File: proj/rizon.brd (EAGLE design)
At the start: 100 x 80 mm, 41 parts, among them J1 PWRJACK5521, P1 ADDR, P2 DATA, P3 CTL, P4 PWR, P5 10k, U1 Z8400, U10 74273PDIP, U11 74138PDIP, U12 74138PDIP, U13 74138PDIP, U14 74138PDIP, U15 74138PDIP, U16 7432PDIP, U17 74138PDIP, U2 AS6C62256PDIP, U3 AS6C62256PDIP, U4 AT28C64BPLCC, U5 AT28C64BPLCC, U6 7432PDIP, U7 7805TO220, U8 7432PDIP, U9 7400PDIP, X1 OSC412.7

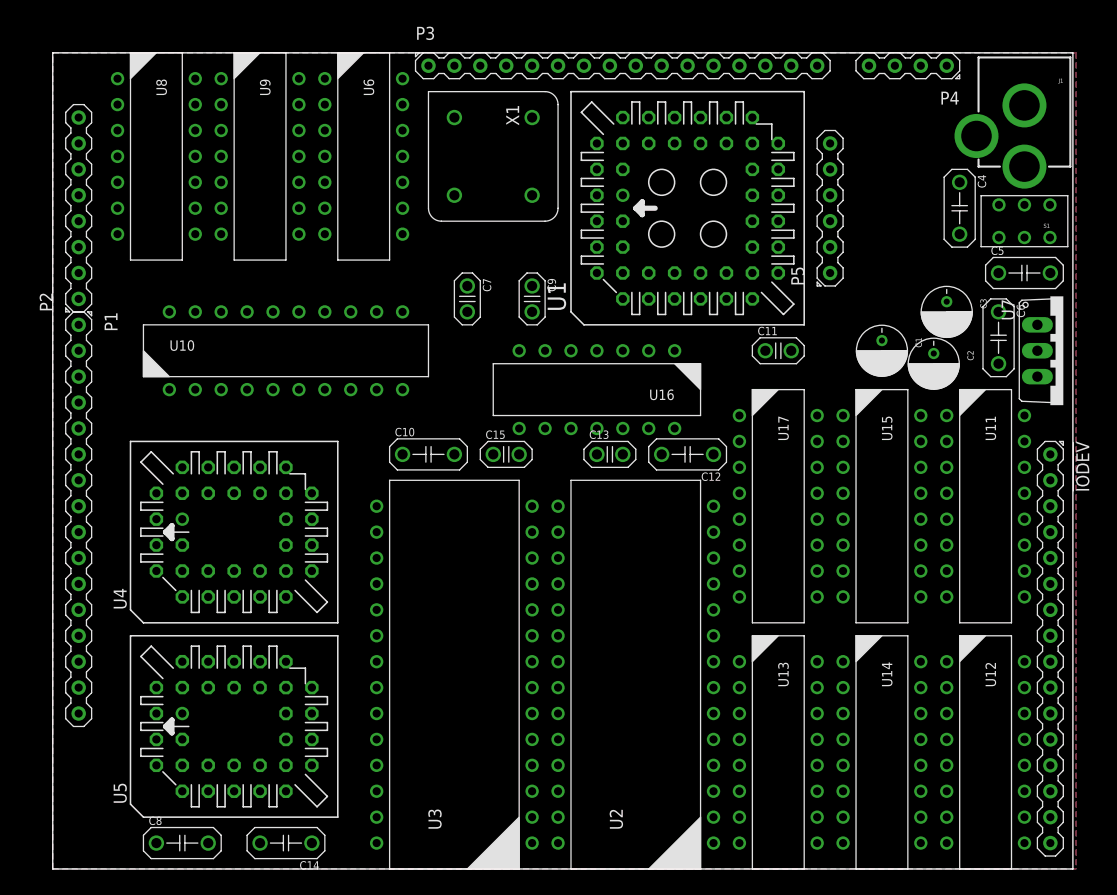
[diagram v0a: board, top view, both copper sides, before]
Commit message: Further designed Rizon board
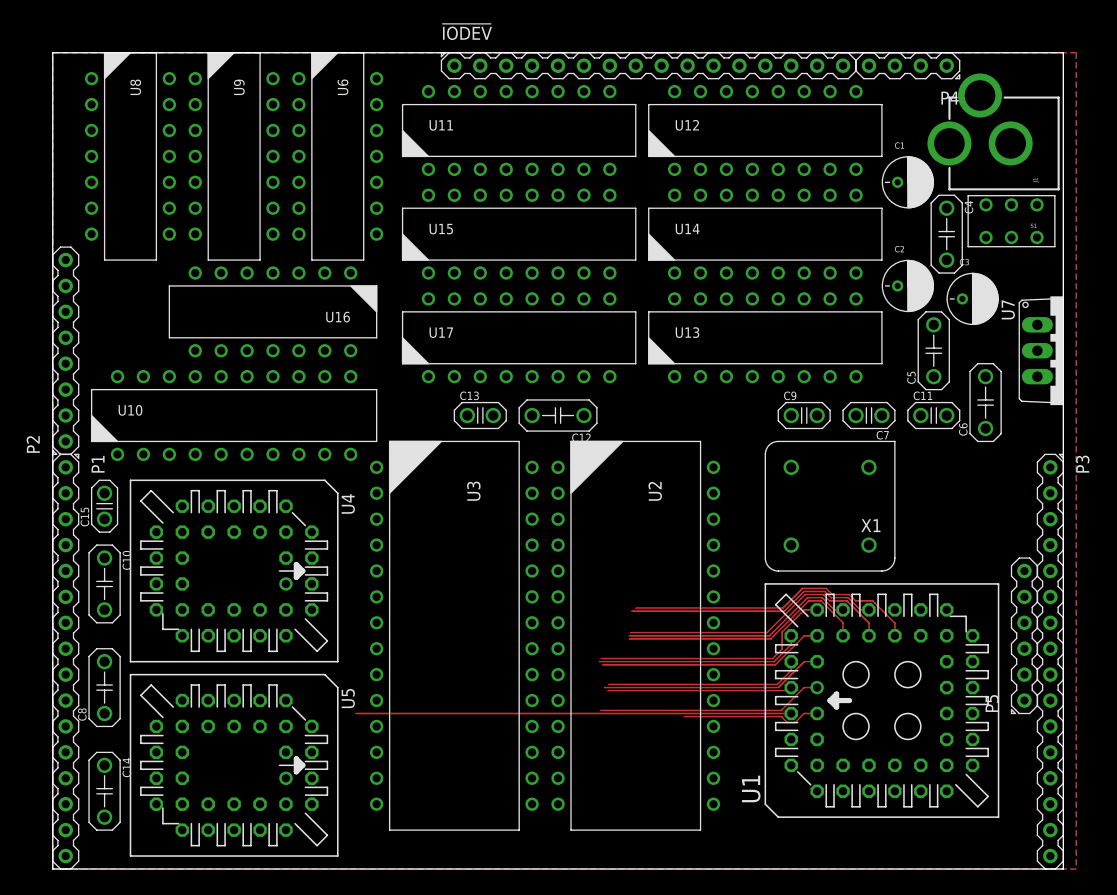
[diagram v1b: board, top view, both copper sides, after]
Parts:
- moved P3 71.9 mm to (97.8, 20.3), turned to 270 degrees
- moved !IODEV 69.4 mm to (58.4, 78.7), turned to 0 degrees
- moved U12 64.7 mm to (69.8, 72.4), turned to 0 degrees
- moved U11 58.7 mm to (45.7, 72.4), turned to 0 degrees
- moved U14 52.1 mm to (69.8, 62.2), turned to 0 degrees
- moved U1 51.9 mm to (81.3, 16.5)
- moved X1 47.6 mm to (76.2, 35.6), turned to 180 degrees
- moved P5 46.0 mm to (95.2, 22.9)
- moved U15 44.4 mm to (45.7, 62.2), turned to 0 degrees
- moved C7 41.0 mm to (80.0, 44.5), turned to 180 degrees
- moved U13 40.7 mm to (69.8, 52.1), turned to 0 degrees
- moved C15 39.7 mm to (5.08, 35.6), turned to 90 degrees
- moved C10 34.2 mm to (5.08, 27.9), turned to 270 degrees
- moved U16 32.7 mm to (21.6, 54.6)
- moved U17 30.3 mm to (45.7, 52.1), turned to 0 degrees
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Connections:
- net !BUSACK: now also P3.7; no longer P3.10
- net !BUSREQ: now also P3.2; no longer P3.12
- net !HALT: now also P3.10; no longer P3.5
- net !INT: now also P3.12; no longer P3.3
- net !IORQ: now also P3.8, U12.P$5; no longer P3.7, U12.P$4
- net !IO_SELECT_BANK1: now also U12.P$4; no longer U12.P$5
- net !M1: now also P3.1; no longer P3.13
- net !MREQ: now also P3.11; no longer P3.6
- net !NMI: now also P3.13; no longer P3.4
- net !RD: now also P3.9; no longer P3.8
- net !RESET: now also P3.3, P5.5; no longer P3.15, P5.4
- net !RFSH: now also P3.5; no longer P3.14
- net !WAIT: now also P3.4, P5.4; no longer P3.11, P5.5
- net !WR: now also P3.6; no longer P3.9
- net CLK: now also P3.15; no longer P3.1
- net GND: now also P3.14; no longer P3.2
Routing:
- net ADDR12: track 0.00 -> 42.7 mm
- net ADDR0: track 0.00 -> 28.9 mm
- net ADDR2: track 0.00 -> 27.3 mm
- net ADDR1: track 0.00 -> 24.8 mm
- net ADDR4: track 0.00 -> 24.7 mm
- net ADDR5: track 0.00 -> 24.1 mm
- net ADDR3: track 0.00 -> 23.0 mm
- net ADDR7: track 0.00 -> 22.2 mm
- net ADDR11: track 0.00 -> 22.1 mm
- net ADDR9: track 0.00 -> 21.9 mm
- net ADDR6: track 0.00 -> 20.3 mm
- net ADDR8: track 0.00 -> 19.3 mm
- net ADDR10: track 0.00 -> 18.1 mm
- net ADDR13: track 0.00 -> 13.6 mm
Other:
- board size 100 x 80 mm -> 99.1 x 80 mm
